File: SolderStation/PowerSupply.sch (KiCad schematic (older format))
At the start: 16 parts

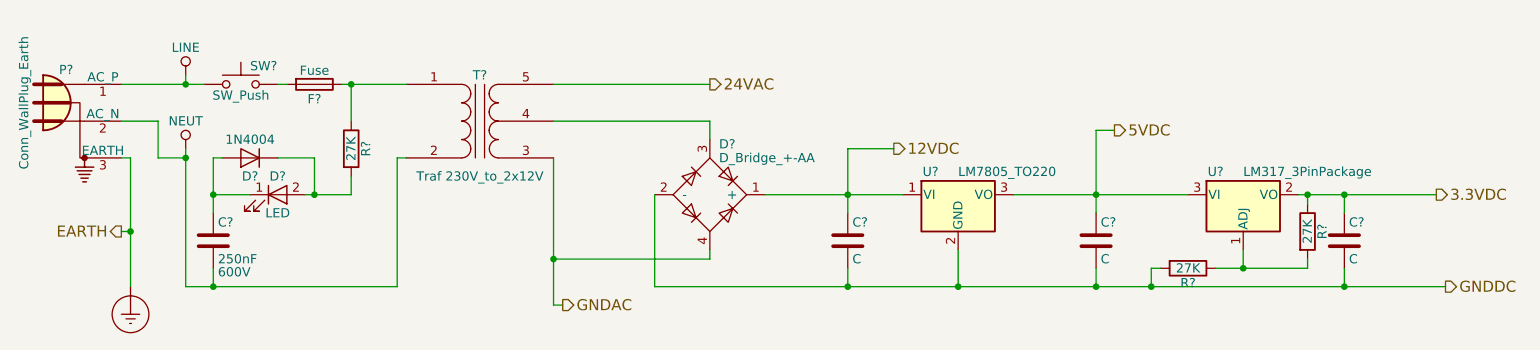
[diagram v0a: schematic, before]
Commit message: Revert "Add files via upload"
This reverts commit 9e82852e4677a33747f2b205dd1fce6c4e717f3a.
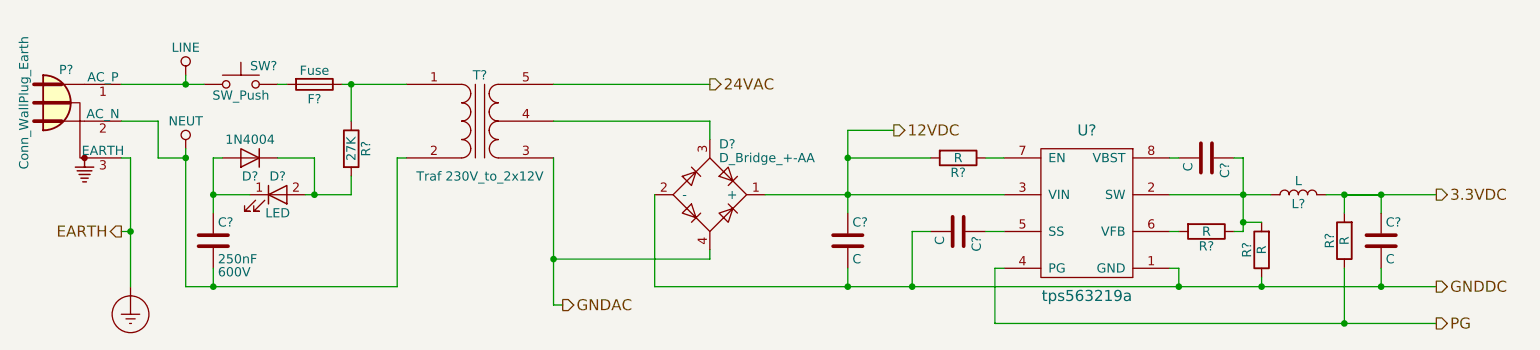
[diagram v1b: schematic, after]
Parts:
- removed C?: C, symbol C
- removed R? (x2): 27K, symbol R
- removed U?: LM7805_TO220, TO_SOT_Packages_THT:TO-220_Vertical, symbol LM7805_TO220
- removed U?: LM317_3PinPackage, symbol LM317_3PinPackage
- added C? (x2): C, symbol C
- added L?: L, symbol L
- added R? (x4): R, symbol R
- added U?: tps563219a, symbol tps563219a
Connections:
- net 12VDC: now also R?.2, U?.3 (VIN)
- net 3.3VDC: now also L?.2, R?.2
- net GNDDC: now also C?.2, R?.1, U?.1 (GND)
- new net: R?.1, U?.7 (EN)
- new net: C?.1, U?.5 (SS)
- new net: C?.1, L?.1, R?.1, R?.2, U?.2 (SW)
- new net: C?.2, U?.8 (VBST)
- new net: R?.2, U?.6 (VFB)
- new net PG: R?.1, U?.4 (PG)
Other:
- moved on the sheet: C?
